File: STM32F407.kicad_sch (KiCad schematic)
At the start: 26 parts, among them J901 UART_CONN, J902 CAN_CONN, SW901 SW_SPDT, U901 STM32F407VGTx, Y901 8MHz

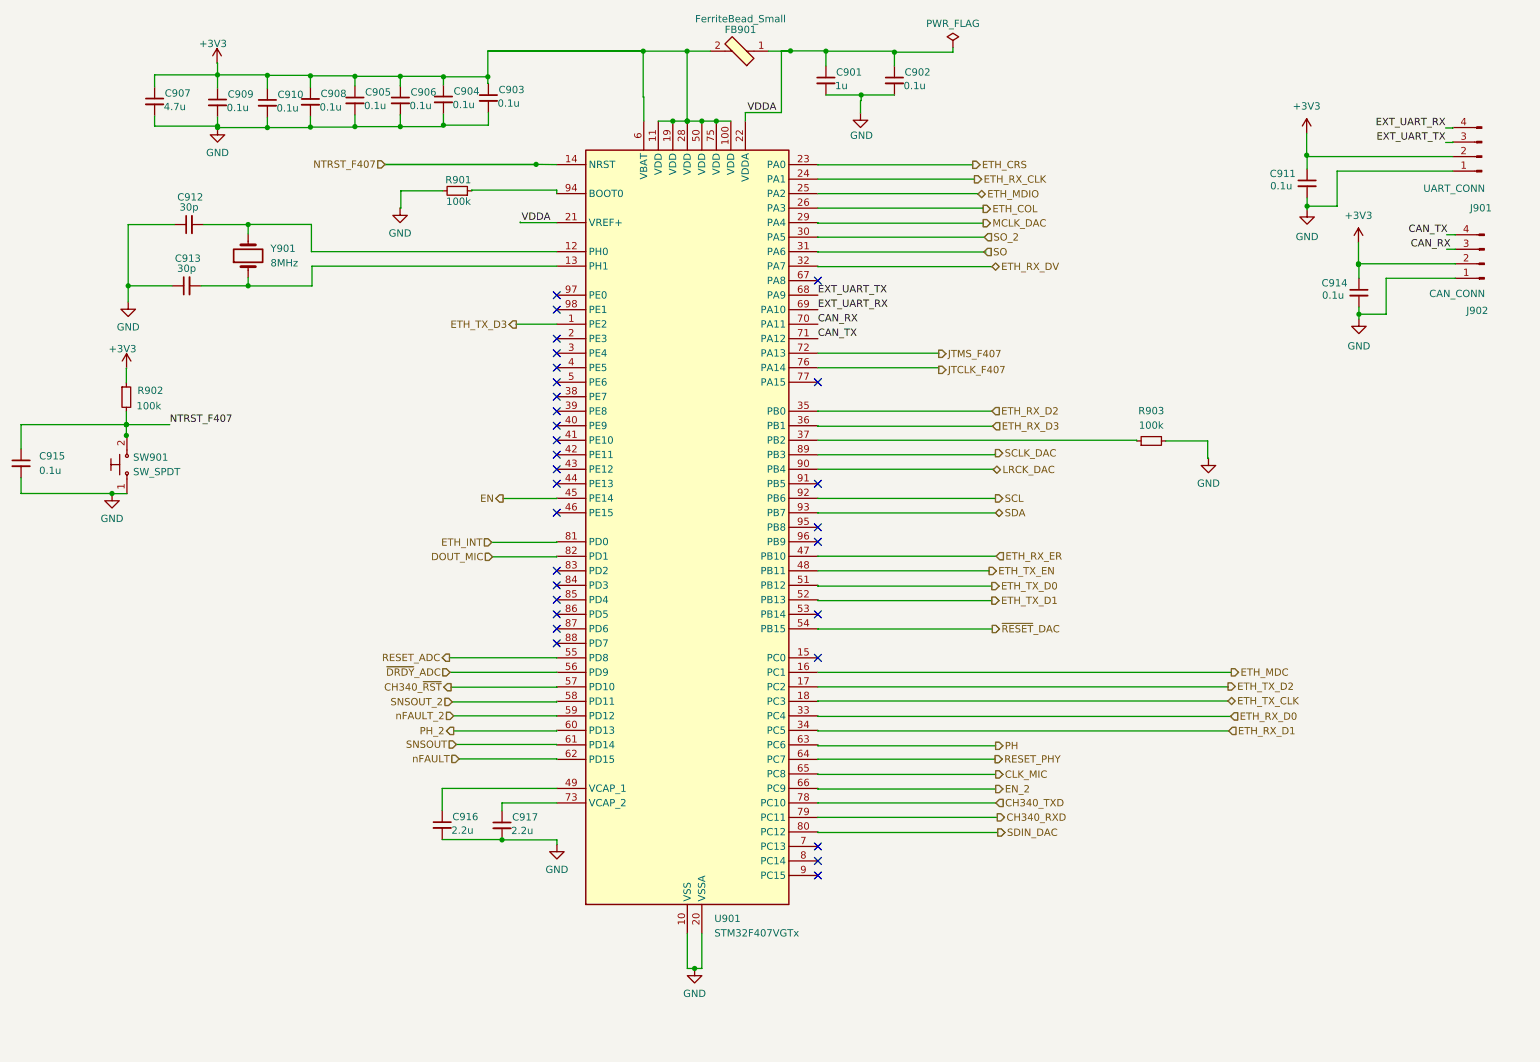
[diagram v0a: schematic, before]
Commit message: schematic pages are reviewed
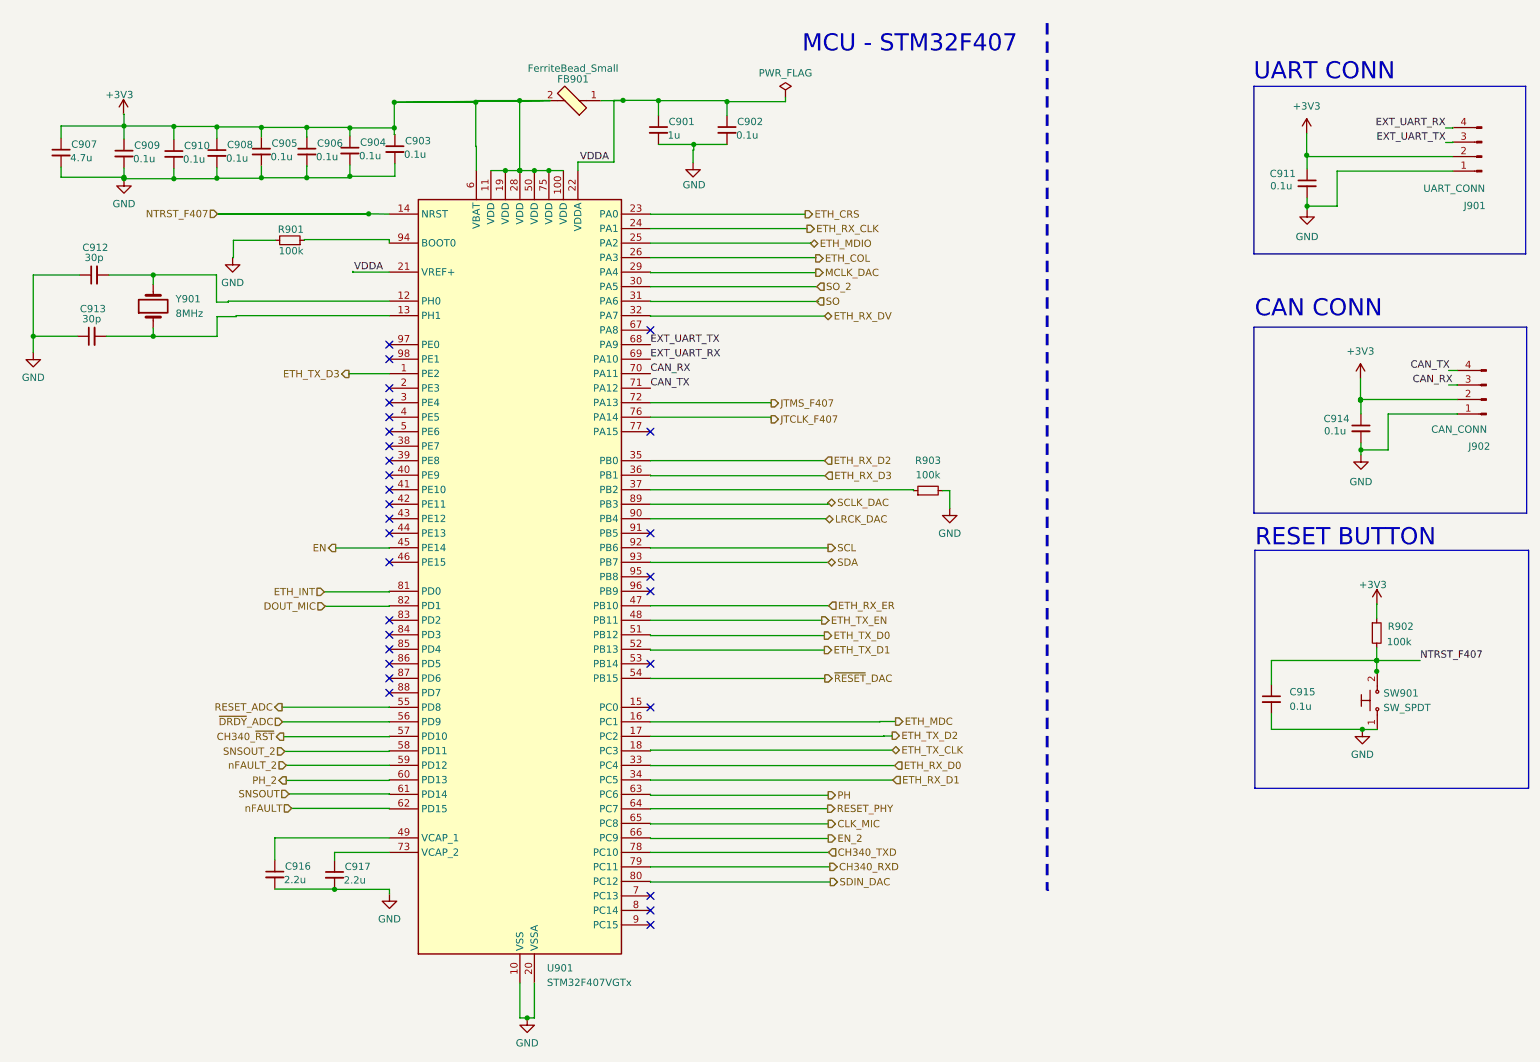
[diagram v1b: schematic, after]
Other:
- note added: "CAN CONN"
- note added: "MCU - STM32F407"
- note added: "RESET BUTTON"
- note added: "UART CONN"
- moved on the sheet: C901, C902, C903, C904, C905, C906, C907, C908, C909, C910, C912, C913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
